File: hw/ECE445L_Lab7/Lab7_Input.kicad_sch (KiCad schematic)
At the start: 5 parts, among them SW1 UP, SW2 DOWN, SW3 LEFT, SW4 RIGHT, SW5 MODE

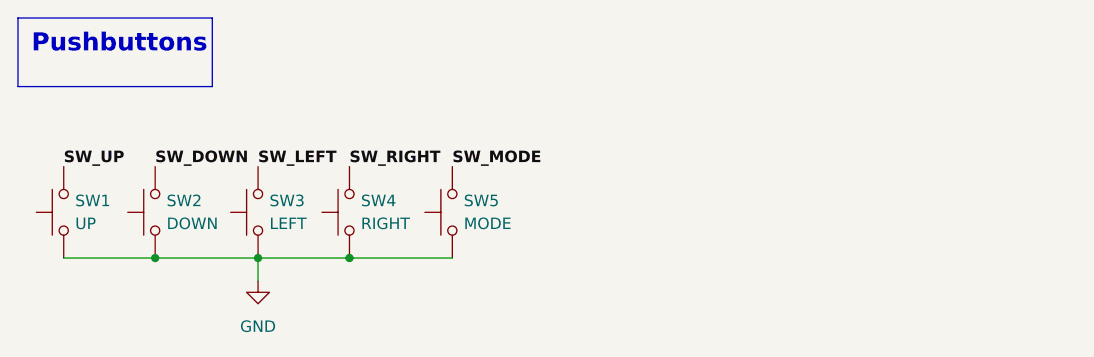
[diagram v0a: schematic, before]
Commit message: work on schem
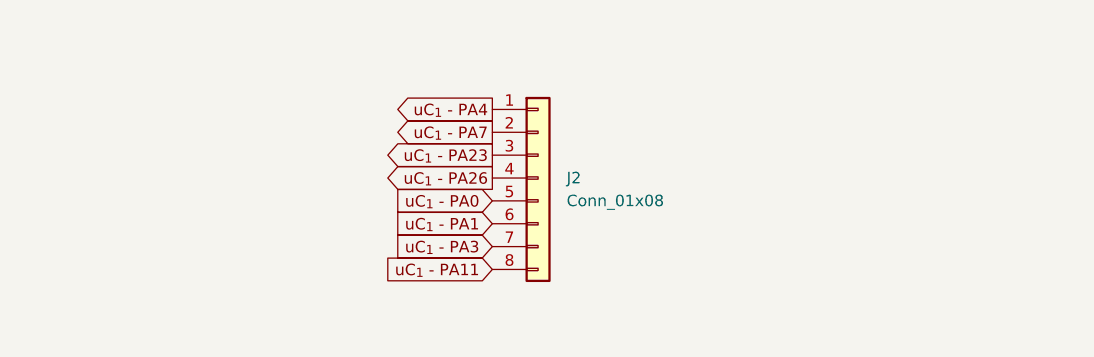
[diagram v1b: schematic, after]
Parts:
- removed SW1: UP, ECE445L:SW_PUSH_6mm, symbol ECE445L:SW_Push
- removed SW2: DOWN, ECE445L:SW_PUSH_6mm, symbol ECE445L:SW_Push
- removed SW3: LEFT, ECE445L:SW_PUSH_6mm, symbol ECE445L:SW_Push
- removed SW4: RIGHT, ECE445L:SW_PUSH_6mm, symbol ECE445L:SW_Push
- removed SW5: MODE, ECE445L:SW_PUSH_6mm, symbol ECE445L:SW_Push
- added J2: Conn_01x08, symbol Connector_Generic:Conn_01x08
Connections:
- new net uC_{1} - PA0: J2.5 (Pin_5)
- new net uC_{1} - PA1: J2.6 (Pin_6)
- new net uC_{1} - PA11: J2.8 (Pin_8)
- new net uC_{1} - PA23: J2.3 (Pin_3)
- new net uC_{1} - PA26: J2.4 (Pin_4)
- new net uC_{1} - PA3: J2.7 (Pin_7)
- new net uC_{1} - PA4: J2.1 (Pin_1)
- new net uC_{1} - PA7: J2.2 (Pin_2)

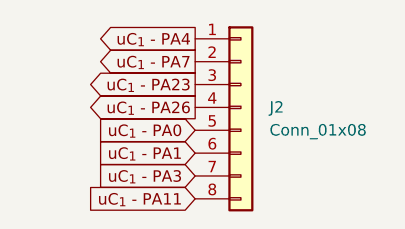
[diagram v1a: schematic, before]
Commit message: more updates
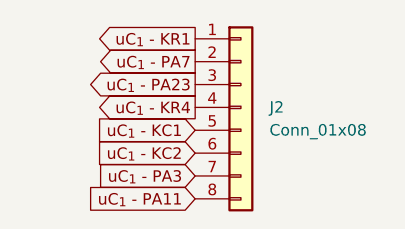
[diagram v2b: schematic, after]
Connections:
- net uC_{1} - PA0 renamed uC_{1} - KC1
- net uC_{1} - PA1 renamed uC_{1} - KC2
- net uC_{1} - PA26 renamed uC_{1} - KR4
- net uC_{1} - PA4 renamed uC_{1} - KR1
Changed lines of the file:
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@@
 	(generator_version "10.0")
 	(paper "A4")
-	(global_label "uC_{1} - PA4"
+	(global_label "uC_{1} - KR1"
 		(shape output)
 		(at 87.63 40.005 180)
@@
 		)
 		(property "Intersheetrefs" "${INTERSHEET_REFS}"
-			(at 74.1825 40.005 0)
+			(at 74.0011 40.005 0)
 			(hide yes)
 			(show_name no)
@@
 		)
 	)
-	(global_label "uC_{1} - PA1"
+	(global_label "uC_{1} - KC2"
 		(shape input)
 		(at 87.63 52.705 180)
@@
 		)
 		(property "Intersheetrefs" "${INTERSHEET_REFS}"
-			(at 74.1825 52.705 0)
+			(at 74.0011 52.705 0)
 			(hide yes)
 			(show_name no)
@@
 		)
 	)
-	(global_label "uC_{1} - PA0"
+	(global_label "uC_{1} - KC1"
 		(shape input)
 		(at 87.63 50.165 180)
@@
 		)
 		(property "Intersheetrefs" "${INTERSHEET_REFS}"
-			(at 74.1825 50.165 0)
+			(at 74.0011 50.165 0)
 			(hide yes)
 			(show_name no)
@@
 		)
 	)
-	(global_label "uC_{1} - PA26"
+	(global_label "uC_{1} - KR4"
 		(shape output)
 		(at 87.63 47.625 180)
@@
 		)
 		(property "Intersheetrefs" "${INTERSHEET_REFS}"
-			(at 72.973 47.625 0)
+			(at 74.0011 47.625 0)
 			(hide yes)
 			(show_name no)

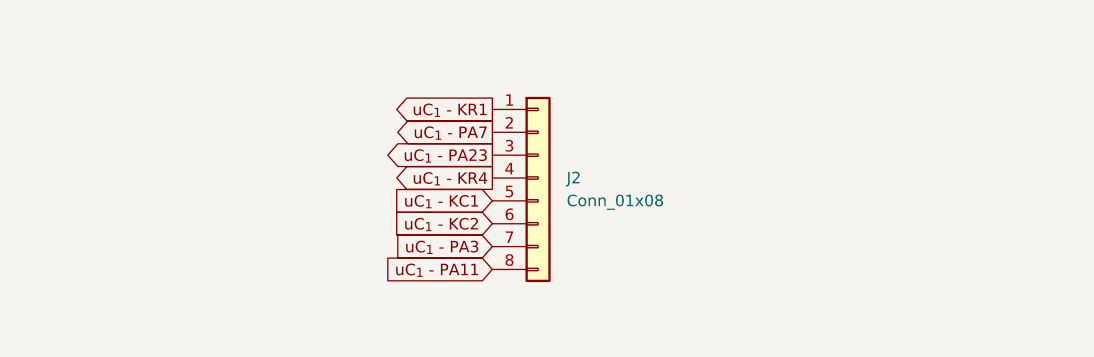
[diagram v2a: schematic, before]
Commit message: mostly finished schem
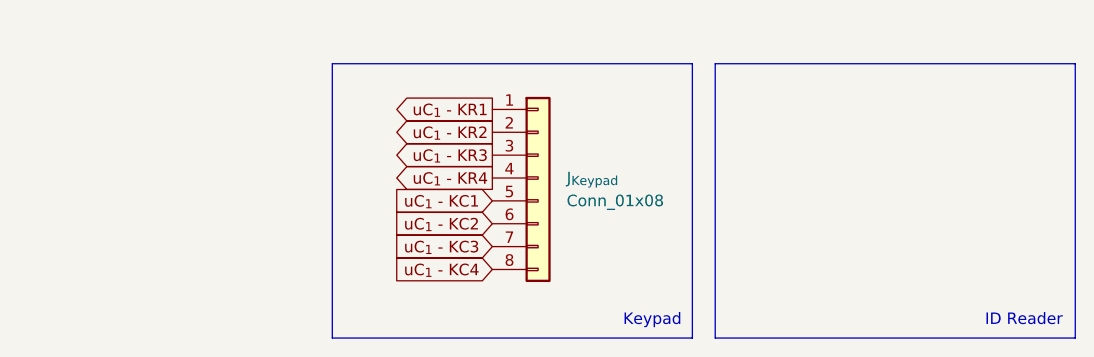
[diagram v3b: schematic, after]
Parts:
- J_{Keypad}: renamed from J2; footprint (none) -> Connector_PinSocket_2.54mm:PinSocket_1x08_P2.54mm_Vertical
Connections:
- net uC_{1} - PA11 renamed uC_{1} - KC4
- net uC_{1} - PA23 renamed uC_{1} - KR3
- net uC_{1} - PA3 renamed uC_{1} - KC3
- net uC_{1} - PA7 renamed uC_{1} - KR2
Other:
- note added: "ID Reader"
- note added: "Keypad"
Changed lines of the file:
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@@
 	(generator_version "10.0")
 	(paper "A4")
+	(rectangle
+		(start 69.85 34.925)
+		(end 109.855 65.405)
+		(stroke
+			(width 0)
+			(type default)
+		)
+		(fill
+			(type none)
+		)
+	)
+	(rectangle
+		(start 112.395 34.925)
+		(end 152.4 65.405)
+		(stroke
+			(width 0)
+			(type default)
+		)
+		(fill
+			(type none)
+		)
+	)
+	(text "ID Reader"
+		(exclude_from_sim no)
+		(at 146.685 63.5 0)
+		(effects
+			(font
+				(size 1.27 1.27)
+			)
+		)
+	)
+	(text "Keypad"
+		(exclude_from_sim no)
+		(at 105.41 63.5 0)
+		(effects
+			(font
+				(size 1.27 1.27)
+			)
+		)
+	)
 	(global_label "uC_{1} - KR1"
 		(shape output)
@@
 		)
 	)
-	(global_label "uC_{1} - PA23"
+	(global_label "uC_{1} - KR3"
 		(shape output)
 		(at 87.63 45.085 180)
@@
 		)
 		(property "Intersheetrefs" "${INTERSHEET_REFS}"
-			(at 72.973 45.085 0)
-			(hide yes)
-			(show_name no)
-			(do_not_autoplace no)
-			(effects
-				(font
-					(size 1.27 1.27)
-				)
-				(justify right)
-			)
-		)
-	)
-	(global_label "uC_{1} - PA11"
+			(at 74.0011 45.085 0)
+			(hide yes)
+			(show_name no)
+			(do_not_autoplace no)
+			(effects
+				(font
+					(size 1.27 1.27)
+				)
+				(justify right)
+			)
+		)
+	)
+	(global_label "uC_{1} - KC4"
 		(shape input)
 		(at 87.63 57.785 180)
@@
 		)
 		(property "Intersheetrefs" "${INTERSHEET_REFS}"
-			(at 72.973 57.785 0)
+			(at 74.0011 57.785 0)
 			(hide yes)
 			(show_name no)
@@
 		)
 	)
-	(global_label "uC_{1} - PA7"
+	(global_label "uC_{1} - KR2"
 		(shape output)
 		(at 87.63 42.545 180)
@@
 		)
 		(property "Intersheetrefs" "${INTERSHEET_REFS}"
-			(at 74.1825 42.545 0)
+			(at 74.0011 42.545 0)
 			(hide yes)
 			(show_name no)
@@
 		)
 	)
-	(global_label "uC_{1} - PA3"
+	(global_label "uC_{1} - KC3"
 		(shape input)
 		(at 87.63 55.245 180)
@@
 		)
 		(property "Intersheetrefs" "${INTERSHEET_REFS}"
-			(at 74.1825 55.245 0)
+			(at 74.0011 55.245 0)
 			(hide yes)
 			(show_name no)
@@
 		(dnp no)
 		(fields_autoplaced yes)
-		(property "Reference" "J2"
+		(property "Reference" "J_{Keypad}"
 			(at 95.885 47.6249 0)
 			(show_name no)
@@
 			)
 		)
-		(property "Footprint" ""
+		(property "Footprint" "Connector_PinSocket_2.54mm:PinSocket_1x08_P2.54mm_Vertical"
 			(at 92.71 47.625 0)
 			(hide yes)
@@
 			(project "ECE445L_Lab7"
 				(path "/69b823fd-c065-40ff-9bb9-c5835555f3eb/e9432827-5ece-4de0-90fe-13c05c5c04a5"
-					(reference "J2")
+					(reference "J_{Keypad}")
 					(unit 1)
 				)
